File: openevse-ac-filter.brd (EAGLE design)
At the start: 64.9 x 23.9 mm, 7 parts

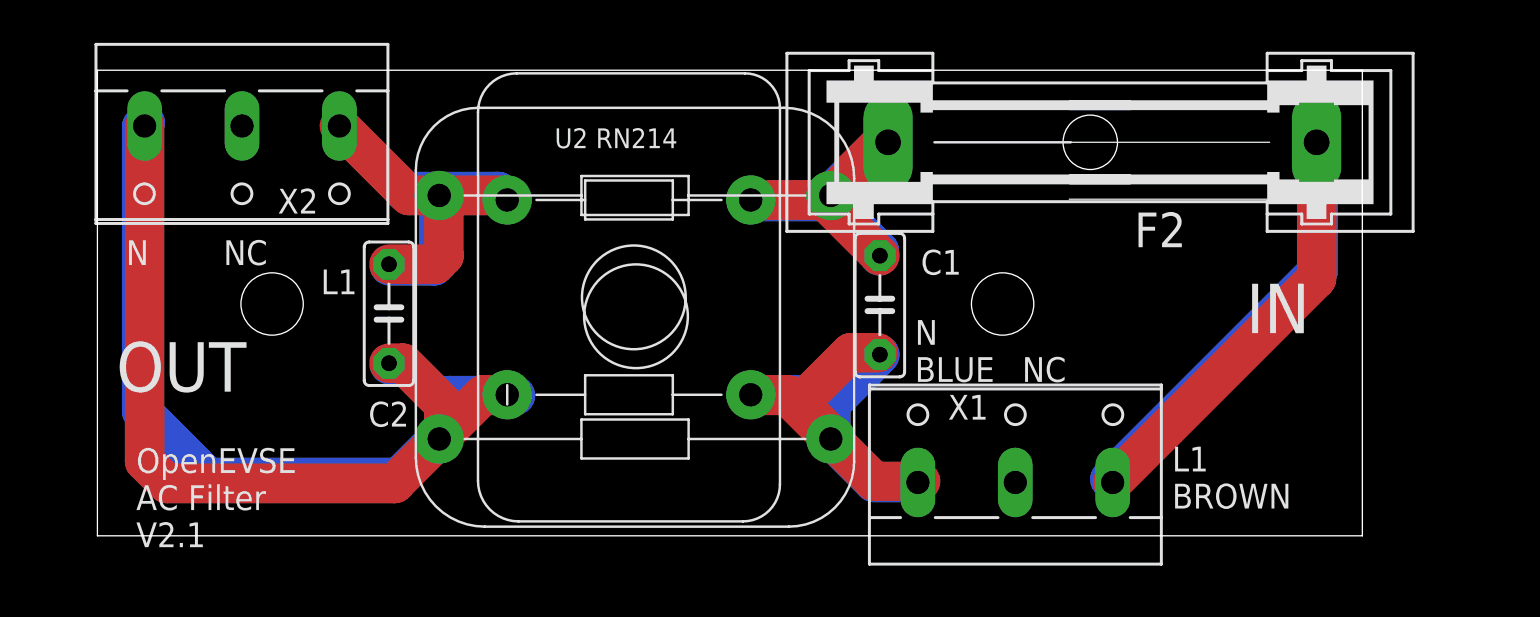
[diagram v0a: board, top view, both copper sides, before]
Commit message: v2.2
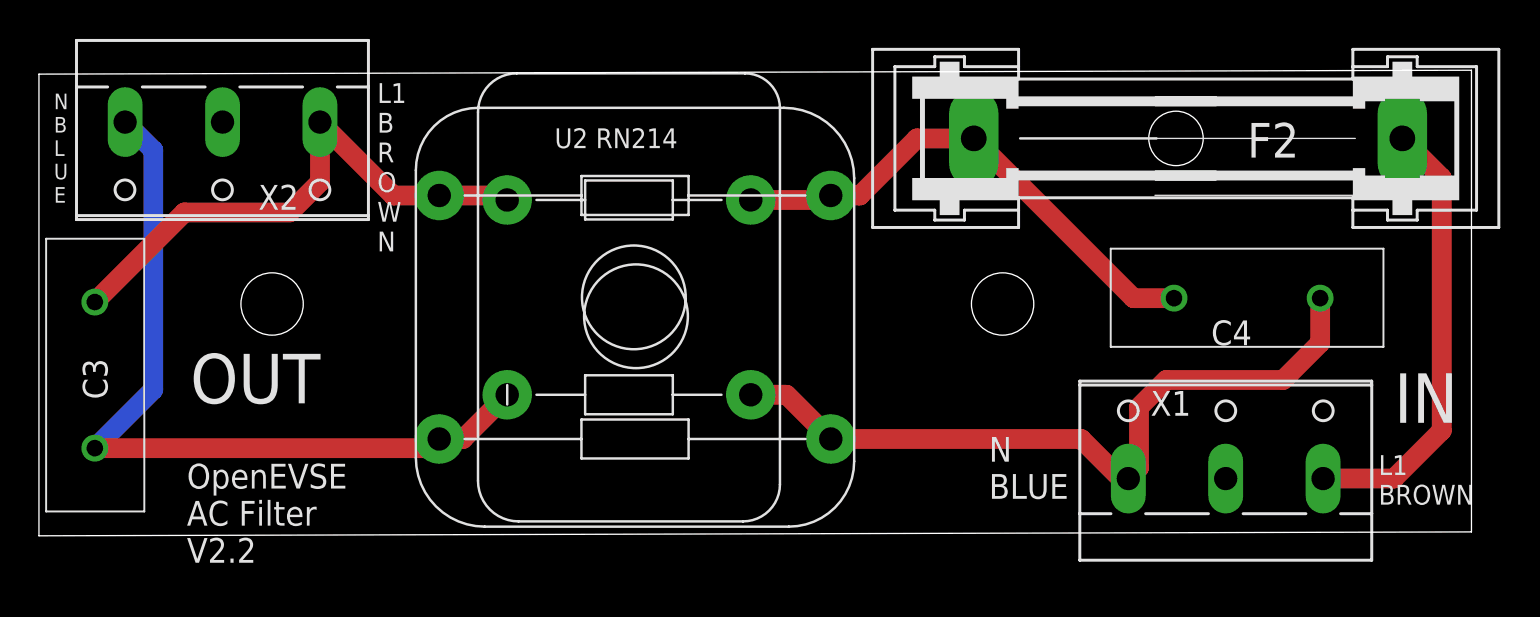
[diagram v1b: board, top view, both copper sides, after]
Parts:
- removed C1: 10F, capacitor-wima:C5B2.5
- removed C2: 10nF, capacitor-wima:C5B2.5
- added C3, C4: DE2F3KY103MA3BM02F, DE2F3KY103MA3BM02F:DE2F3KY103MA3BM02F
- moved X1 10.8 mm to (60.5, 3.83)
- moved F2 4.40 mm to (61.9, 20.0)
- moved X2 1.02 mm to (8.96, 19.5)
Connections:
- removed net N$1: C1.1, U$1.P$4, U$2.P$4, X1.1
- removed net N$2: C1.2, F2.2, U$1.P$2, U$2.P$2
- removed net N$4: C2.2, U$1.P$1, U$2.P$1, X2.1
- new net N$17: C4.2, U$1.P$4, U$2.P$4, X1.1
- new net N$21: C3.1, U$1.P$1, U$2.P$1, X2.1
- new net N$22: C4.1, F2.2, U$1.P$2, U$2.P$2
- net N$3: now also C3.2; no longer C2.1
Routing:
- net N$17: track 0.00 -> 38.4 mm
- net N$19: track 38.2 -> 0.00 mm
- net N$21: track 0.00 -> 28.5 mm
- net N$22: track 0.00 -> 26.4 mm
- net N$1: track 22.3 -> 0.00 mm
- net N$7: track 21.7 -> 0.00 mm
- net N$4: track 16.4 -> 0.00 mm
- net N$2: track 12.5 -> 0.00 mm
- net N$16: track 7.84 -> 0.00 mm
- net N$18: track 7.69 -> 0.00 mm
- net N$20: track 6.61 -> 0.00 mm
- net N$11: track 5.69 -> 0.00 mm
- net N$12: track 5.54 -> 0.00 mm
- net N$13: track 4.42 -> 0.00 mm
- net N$10: track 4.35 -> 0.00 mm
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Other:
- board size 64.9 x 23.9 mm -> 73.5 x 23.9 mm
- board text added: "L1 B R O W N"
- board text added: "N B L U E"
- board text added: "OpenEVSE AC Filter V2.2"
- board text removed: "L1"
- board text removed: "N"
- board text removed: "NC"
- board text removed: "OpenEVSE AC Filter V2.1"
